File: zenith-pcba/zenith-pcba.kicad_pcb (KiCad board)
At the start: 2 copper layers, 2 parts, among them U1 XC7A50T-CSG325, U2 K4B4G1646E-BCNB

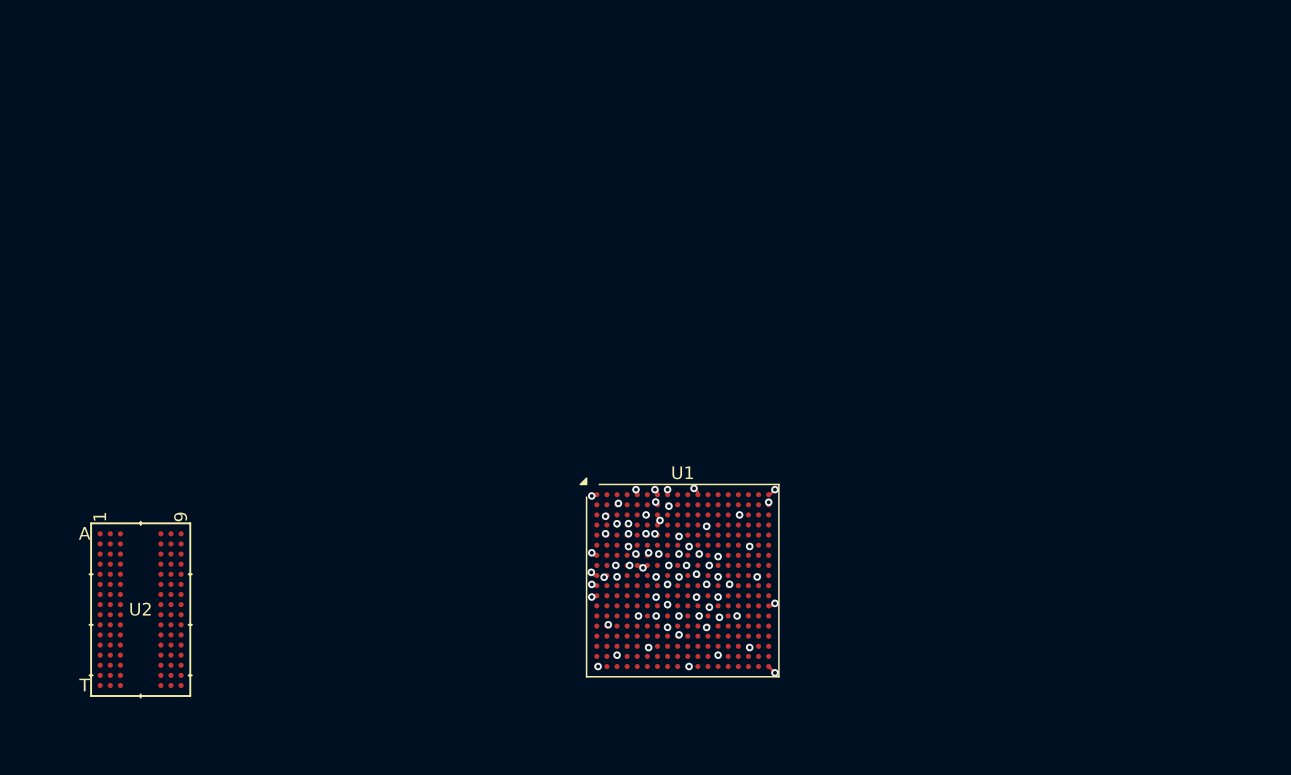
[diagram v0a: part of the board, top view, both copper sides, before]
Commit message: feat(pcba): initial programmer setup
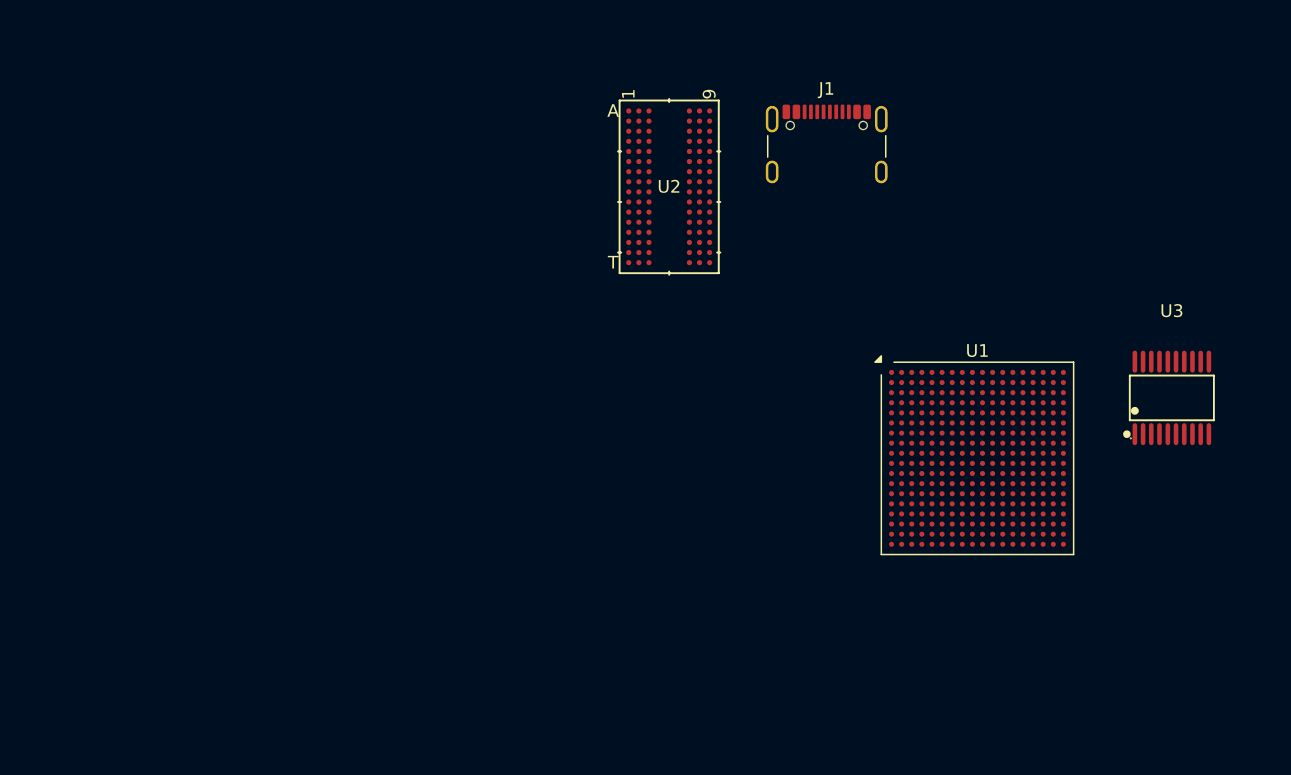
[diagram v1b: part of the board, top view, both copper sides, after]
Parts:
- added J1: USB_C_Receptacle_USB2.0_16P, Connector_USB:USB_C_Receptacle_GCT_USB4105-xx-A_16P_TopMnt_Horizontal, F.Cu at (150.6, 58.3)
- added U3: CH347T, easyeda2kicad:TSSOP-20_L6.5-W4.4-P0.65-LS6.4-BL, F.Cu at (177.9, 77.2)
- moved U2 53.6 mm to (138.1, 60.5)
- moved U1 25.3 mm to (162.5, 82.0)
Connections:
- U1 pad A1: GND -> unconnected-(U1F-GND-PadA1)
- U1 pad A11: GND -> unconnected-(U1F-GND-PadA11)
- U1 pad A18: GND -> unconnected-(U1F-GND-PadA18)
- U1 pad A5: GND -> unconnected-(U1F-GND-PadA5)
- U1 pad A7: GND -> unconnected-(U1F-GND-PadA7)
- U1 pad A8: GND -> unconnected-(U1F-GND-PadA8)
- U1 pad B18: GND -> unconnected-(U1F-GND-PadB18)
- U1 pad B3: GND -> unconnected-(U1F-GND-PadB3)
- U1 pad B7: GND -> unconnected-(U1F-GND-PadB7)
- U1 pad B8: GND -> unconnected-(U1F-GND-PadB8)
- U1 pad C15: GND -> unconnected-(U1F-GND-PadC15)
- U1 pad C2: GND -> unconnected-(U1F-GND-PadC2)
- U1 pad C6: GND -> unconnected-(U1F-GND-PadC6)
- U1 pad C7: GND -> unconnected-(U1F-GND-PadC7)
- U1 pad D12: GND -> unconnected-(U1F-GND-PadD12)
- U1 pad D3: GND -> unconnected-(U1F-GND-PadD3)
- U1 pad D4: GND -> unconnected-(U1F-GND-PadD4)
- U1 pad D7: GND -> unconnected-(U1F-GND-PadD7)
- U1 pad E2: GND -> unconnected-(U1F-GND-PadE2)
- U1 pad E6: GND -> unconnected-(U1F-GND-PadE6)
- U1 pad E7: GND -> unconnected-(U1F-GND-PadE7)
- U1 pad E9: GND -> unconnected-(U1F-GND-PadE9)
- U1 pad F10: GND -> unconnected-(U1F-GND-PadF10)
- U1 pad F16: GND -> unconnected-(U1F-GND-PadF16)
- U1 pad F4: GND -> unconnected-(U1F-GND-PadF4)
- U1 pad F6: GND -> unconnected-(U1F-GND-PadF6)
- U1 pad F8: unconnected-(U1E-TCK_0-PadF8) -> Net-(U1E-TCK_0)
- U1 pad G1: GND -> unconnected-(U1F-GND-PadG1)
- U1 pad G11: GND -> unconnected-(U1F-GND-PadG11)
- U1 pad G13: GND -> unconnected-(U1F-GND-PadG13)
- U1 pad G5: GND -> unconnected-(U1F-GND-PadG5)
- U1 pad G6: GND -> unconnected-(U1F-GND-PadG6)
- U1 pad G7: GND -> unconnected-(U1F-GND-PadG7)
- U1 pad G9: GND -> unconnected-(U1F-GND-PadG9)
- U1 pad H10: GND -> unconnected-(U1F-GND-PadH10)
- U1 pad H12: GND -> unconnected-(U1F-GND-PadH12)
- U1 pad H3: GND -> unconnected-(U1F-GND-PadH3)
- U1 pad H4: GND -> unconnected-(U1F-GND-PadH4)
- U1 pad H5: GND -> unconnected-(U1F-GND-PadH5)
- U1 pad H6: GND -> unconnected-(U1F-GND-PadH6)
- U1 pad H8: GND -> unconnected-(U1F-GND-PadH8)
- U1 pad J1: GND -> unconnected-(U1F-GND-PadJ1)
- U1 pad J11: GND -> unconnected-(U1F-GND-PadJ11)
- U1 pad J13: GND -> unconnected-(U1F-GND-PadJ13)
- U1 pad J17: GND -> unconnected-(U1F-GND-PadJ17)
- U1 pad J2: GND -> unconnected-(U1F-GND-PadJ2)
- U1 pad J3: GND -> unconnected-(U1F-GND-PadJ3)
- U1 pad J7: GND -> unconnected-(U1F-GND-PadJ7)
- U1 pad J9: GND -> unconnected-(U1F-GNDADC_0-PadJ9)
- U1 pad K12: GND -> unconnected-(U1F-GND-PadK12)
- U1 pad K14: GND -> unconnected-(U1F-GND-PadK14)
- U1 pad K4: GND -> unconnected-(U1F-GND-PadK4)
- U1 pad K8: GND -> unconnected-(U1F-GND-PadK8)
- U1 pad L1: GND -> unconnected-(U1F-GND-PadL1)
- U1 pad L11: GND -> unconnected-(U1F-GND-PadL11)
- U1 pad L13: GND -> unconnected-(U1F-GND-PadL13)
- U1 pad L7: GND -> unconnected-(U1F-GND-PadL7)
- U1 pad M12: GND -> unconnected-(U1F-GND-PadM12)
- U1 pad M18: GND -> unconnected-(U1F-GND-PadM18)
- U1 pad M8: GND -> unconnected-(U1F-GND-PadM8)
- U1 pad N11: GND -> unconnected-(U1F-GND-PadN11)
- U1 pad N13: GND -> unconnected-(U1F-GND-PadN13)
- U1 pad N15: GND -> unconnected-(U1F-GND-PadN15)
- U1 pad N5: GND -> unconnected-(U1F-GND-PadN5)
- U1 pad N7: GND -> unconnected-(U1F-GND-PadN7)
- U1 pad N9: GND -> unconnected-(U1F-GND-PadN9)
- U1 pad P12: GND -> unconnected-(U1F-GND-PadP12)
- U1 pad P2: GND -> unconnected-(U1F-GND-PadP2)
- U1 pad P8: GND -> unconnected-(U1F-GND-PadP8)
- U1 pad R8: unconnected-(U1E-TMS_0-PadR8) -> Net-(U1E-TMS_0)
- U1 pad R9: GND -> unconnected-(U1F-GND-PadR9)
- U1 pad T16: GND -> unconnected-(U1F-GND-PadT16)
- U1 pad T6: GND -> unconnected-(U1F-GND-PadT6)
- U1 pad T8: unconnected-(U1E-TDO_0-PadT8) -> Net-(U1E-TDO_0)
- U1 pad T9: unconnected-(U1E-TDI_0-PadT9) -> Net-(U1E-TDI_0)
- U1 pad U13: GND -> unconnected-(U1F-GND-PadU13)
- U1 pad U3: GND -> unconnected-(U1F-GND-PadU3)
- U1 pad V1: GND -> unconnected-(U1F-GND-PadV1)
- U1 pad V10: GND -> unconnected-(U1F-GND-PadV10)
- U1 pad V18: GND -> unconnected-(U1F-GND-PadV18)
- U2 pad A9: /Root/GND -> unconnected-(U2-VSS-PadA9)
- U2 pad T1: /Root/GND -> unconnected-(U2-VSS-PadT1)
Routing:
- net GND: track 15.1 -> 0.00 mm, vias 72 -> 0
- net unconnected-(U1B-IO_L3N_T0_DQS_34-PadK1): track 0.44 -> 0.00 mm, vias 1 -> 0
- net unconnected-(U1C-MGTPRXP0_216-PadE4): track 0.15 -> 0.00 mm, vias 1 -> 0
- added copper zone on B.Cu, net (none)
- removed copper zone on B.Cu, net GND
